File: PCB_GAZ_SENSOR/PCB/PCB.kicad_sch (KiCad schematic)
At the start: 24 parts, among them J0 Conn_01x03_Female, J1 Alimentation externe Resistan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, P1 Power, P2 Analog, P3 Digital, P4 Digital, P5 CONN_01X01, P6 CONN_01X01, P7 CONN_01X01, P8 CONN_01X01, SW0 SW_DPDT_x2, U0 LTC1050, U1 RN2483_Breakout

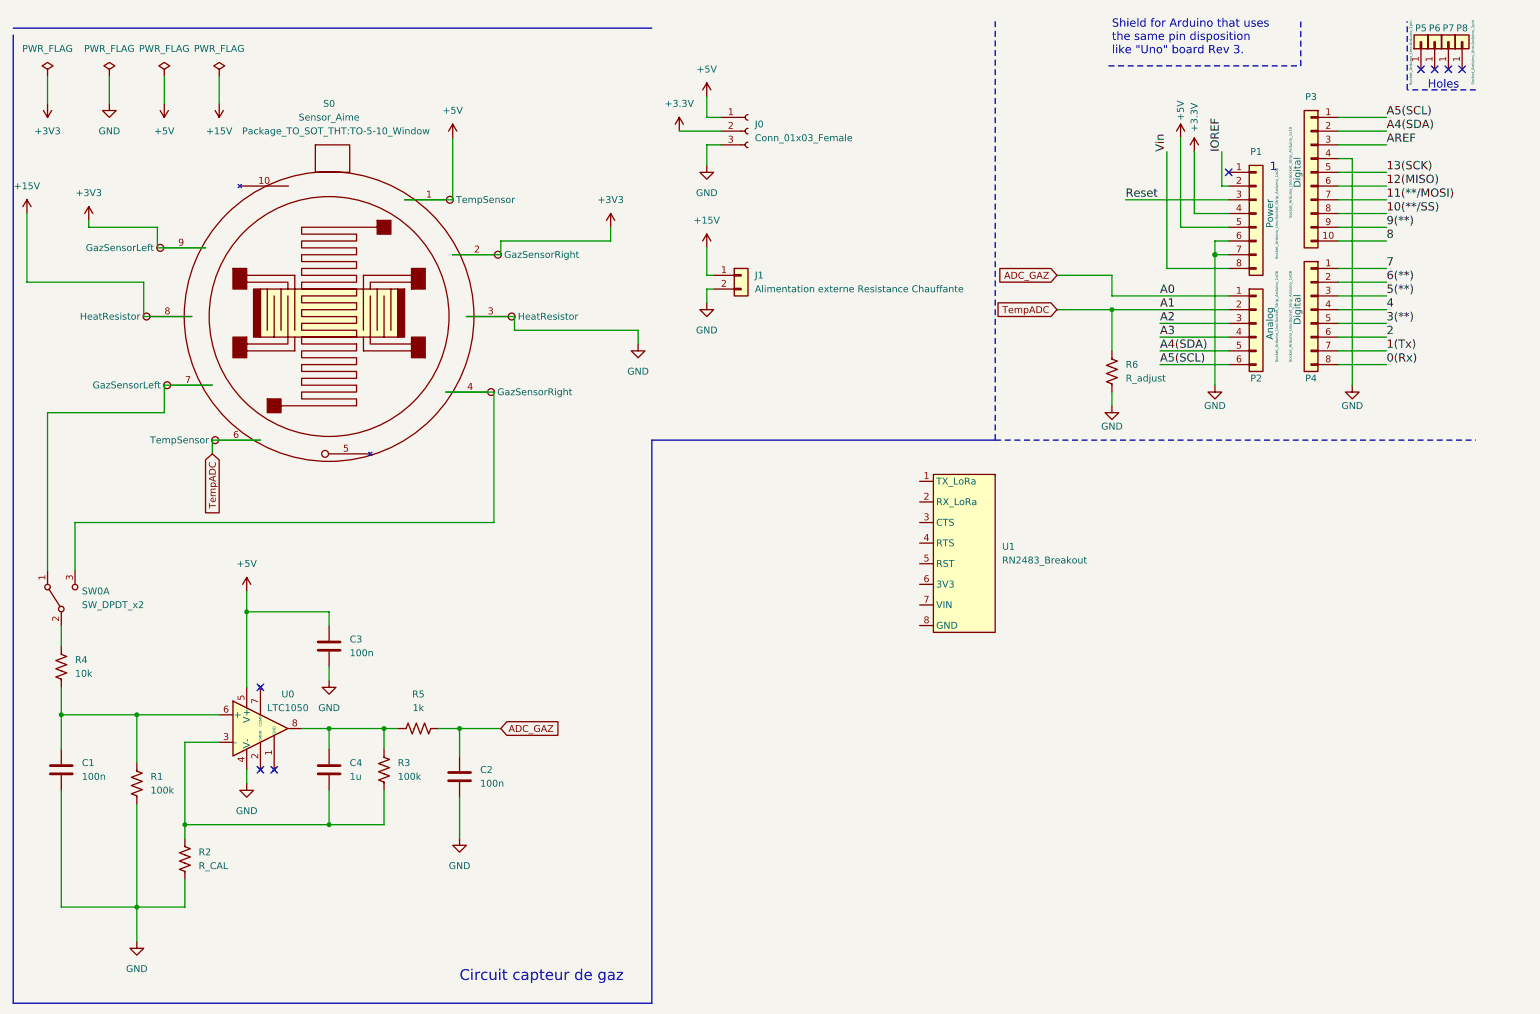
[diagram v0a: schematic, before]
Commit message: final version
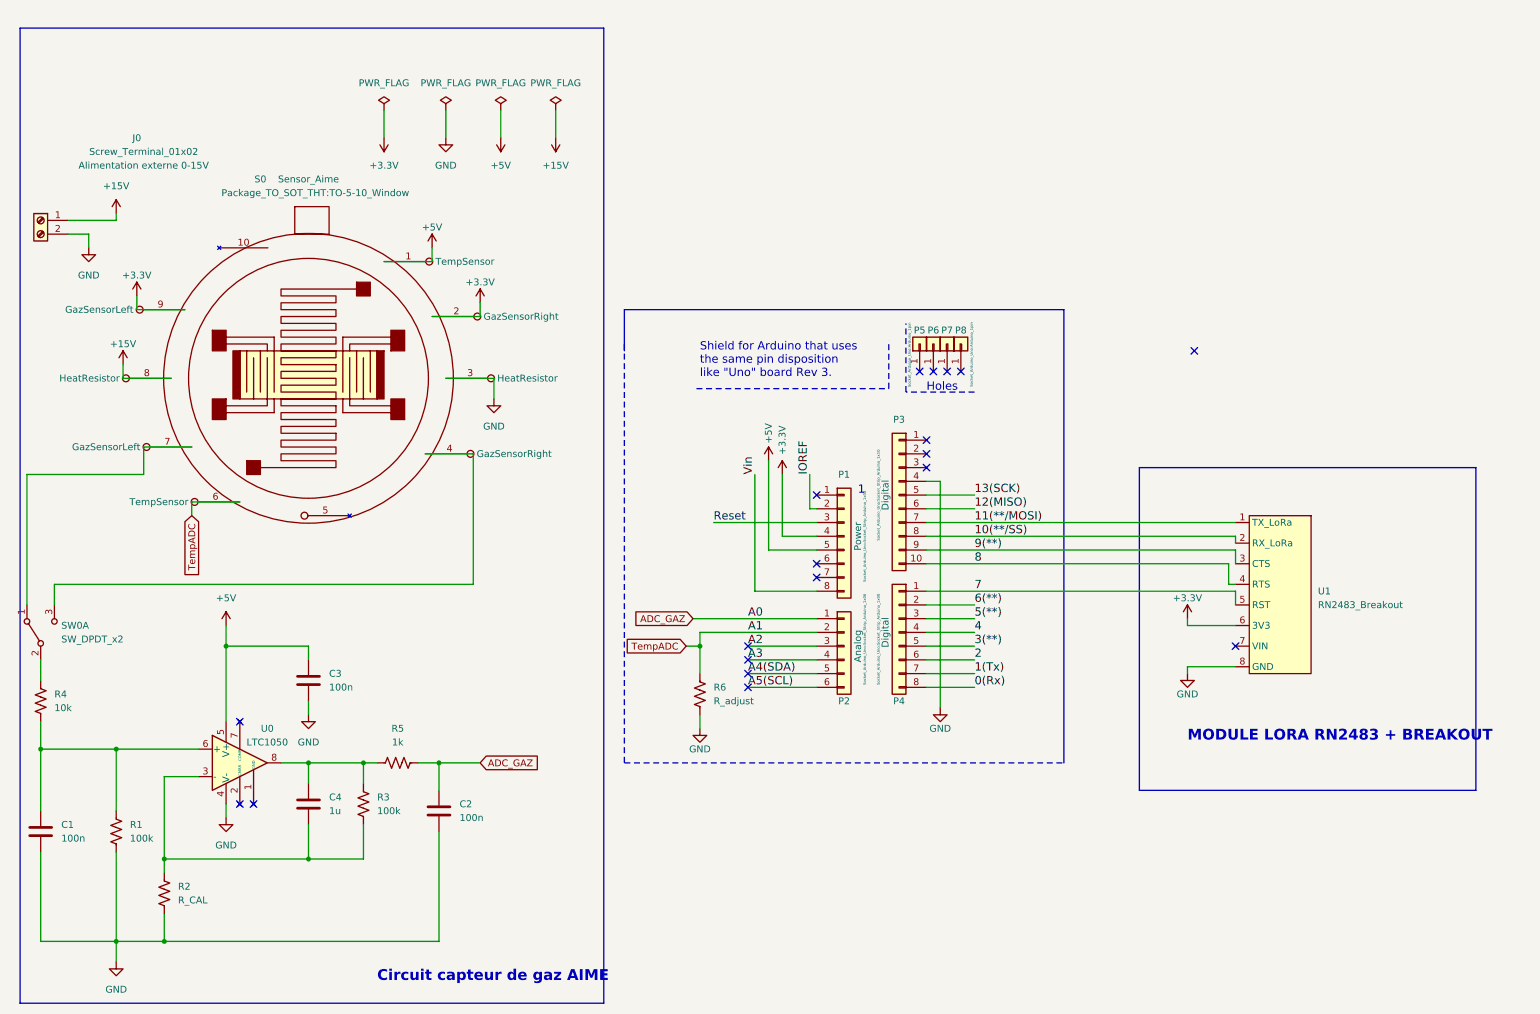
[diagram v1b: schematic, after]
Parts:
- removed J0: Conn_01x03_Female, Connector_PinSocket_2.54mm:PinSocket_1x03_P2.54mm_Vertical, symbol Connector:Conn_01x03_Female
- removed J1: Alimentation externe Resistance Chauffante, Connector_PinHeader_2.54mm:PinHeader_1x02_P2.54mm_Vertical, symbol Connector_Generic:Conn_01x02
- added J0: Screw_Terminal_01x02, TerminalBlock_Phoenix:TerminalBlock_Phoenix_MKDS-1,5-2-5.08_1x02_P5.08mm_Horizontal, symbol Connector:Screw_Terminal_01x02
- C1, C2, C3, C4: footprint (none) -> Capacitor_THT:CP_Radial_D5.0mm_P2.50mm
- R1, R2, R3, R4, R5, R6: footprint (none) -> Resistor_THT:R_Axial_DIN0204_L3.6mm_D1.6mm_P7.62mm_Horizontal
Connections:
- net +15V: now also J0.1 (Pin_1)
- net +3V3: now also U1.6 (3V3)
- net 10(**/SS): now also U1.2 (RX_LoRa)
- net 11(**/MOSI): now also U1.1 (TX_LoRa)
- net 7: now also U1.5 (RST)
- net 8: now also U1.4 (RTS)
- net 9(**): now also U1.3 (CTS)
- net A4(SDA): no longer P3.2 (Pin_2)
- net A5(SCL): no longer P3.1 (Pin_1)
- net GND: now also U1.8 (GND), J0.2 (Pin_2); no longer P1.6 (Pin_6), P1.7 (Pin_7)
- net AREF: no longer names the net of P3.3 (Pin_3)
- no-connect marks 8 -> 19
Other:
- note added: "Circuit capteur de gaz AIME"
- note added: "MODULE LORA RN2483 + BREAKOUT"
- note removed: "Circuit capteur de gaz"
- title: PCB GAZ SENSOR -> SCHEMATIQUE GAZ SENSOR
- moved on the sheet: C1, C2, C3, C4, P1, P2, P3, P4, P5, P6, P7, P8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
